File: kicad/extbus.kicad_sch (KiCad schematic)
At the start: 19 parts, among them J20 Spare resistors, J21 Power bar, J22 Spare resistors, J23 BUS Slot 2, J24 BUS Slot 1

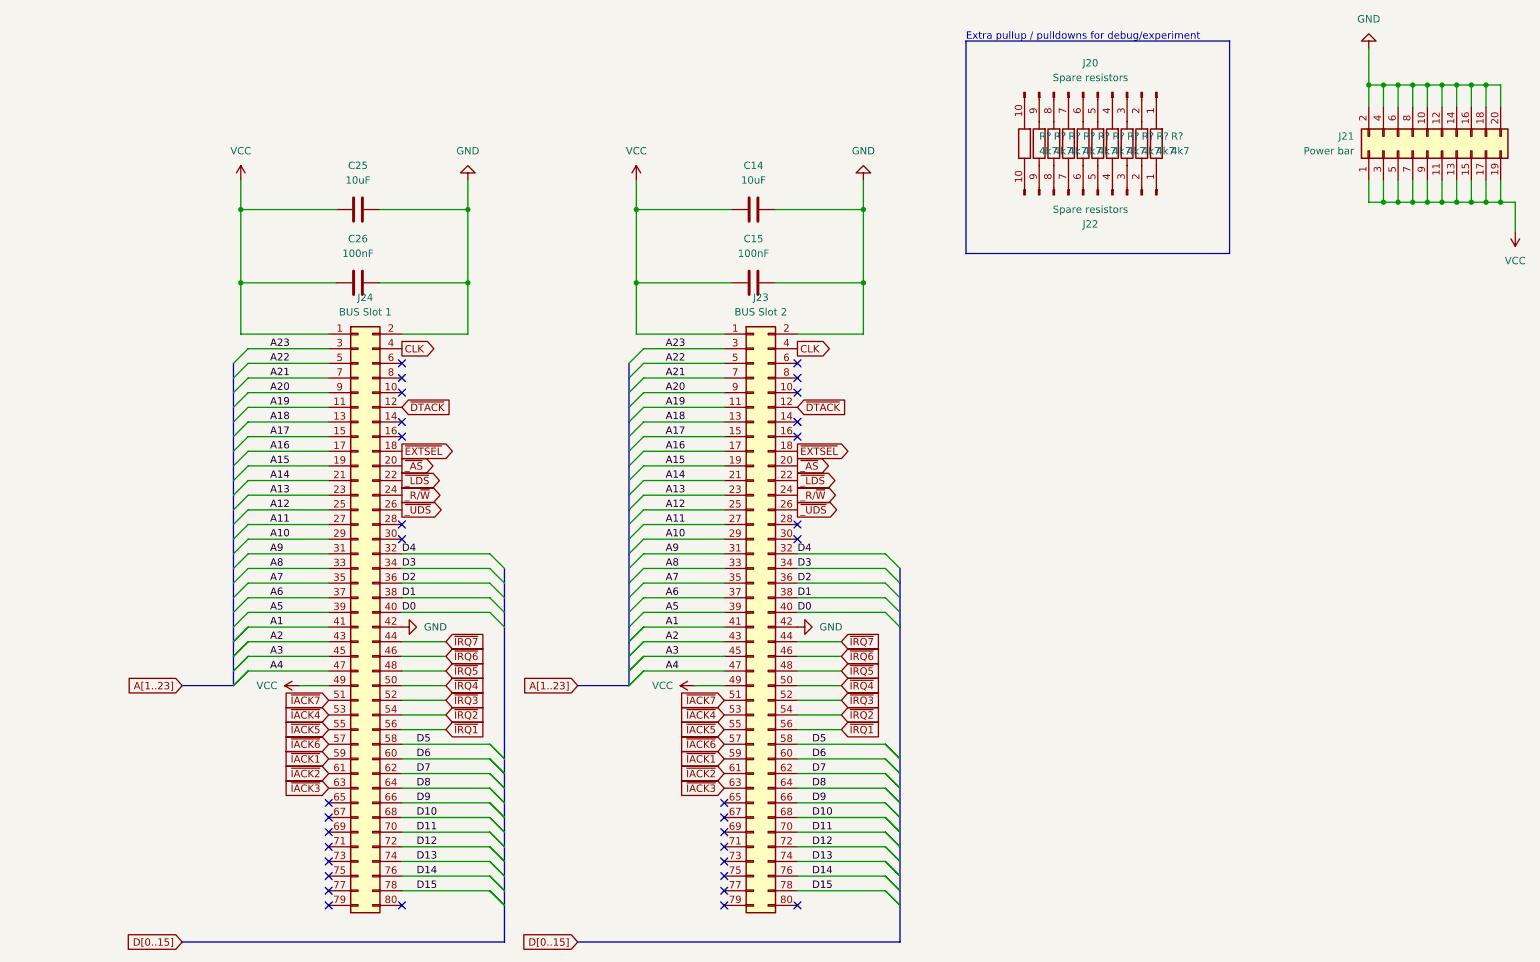
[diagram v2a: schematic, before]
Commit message: fiddlign with placement
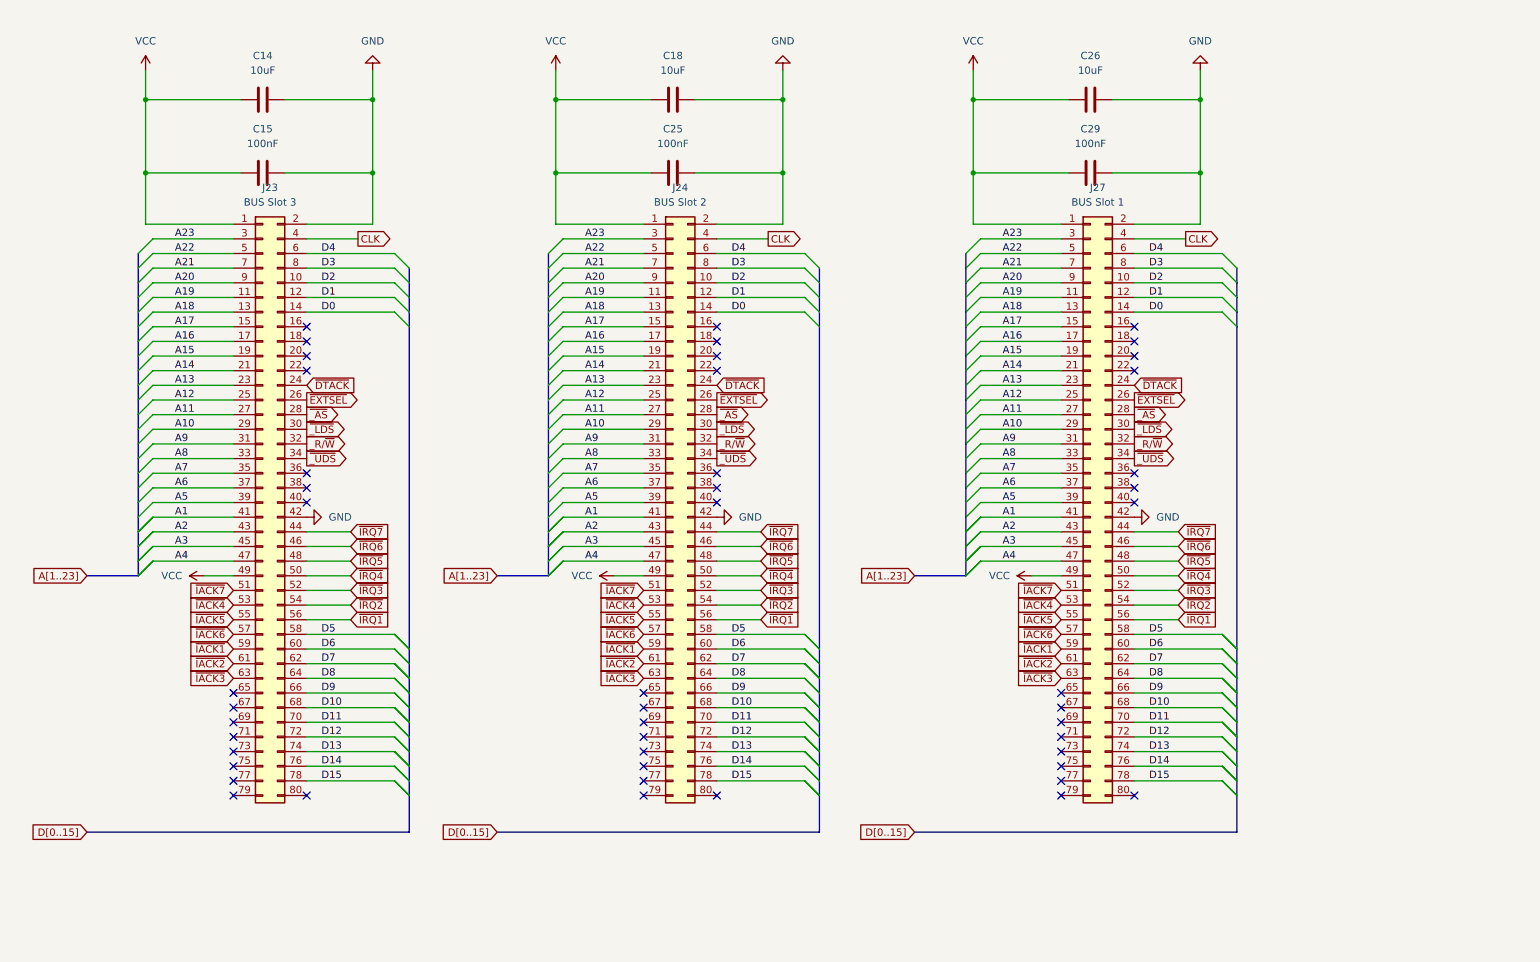
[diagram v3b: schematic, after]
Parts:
- removed J20, J22: Spare resistors, Connector_PinSocket_2.54mm:PinSocket_1x10_P2.54mm_Vertical, symbol Connector:Conn_01x10_Pin
- removed J21: Power bar, Connector_PinSocket_2.54mm:PinSocket_2x10_P2.54mm_Vertical, symbol Connector_Generic:Conn_02x10_Odd_Even
- removed R? (x10): 4k7, Resistor_THT:R_Axial_DIN0207_L6.3mm_D2.5mm_P10.16mm_Horizontal, symbol Device:R
- added C18: 10uF, Capacitor_THT:CP_Radial_D5.0mm_P2.50mm, symbol Device:C
- added C29: 100nF, Capacitor_THT:CP_Radial_D5.0mm_P2.50mm, symbol Device:C
- added J27: BUS Slot 1, Connector_PinSocket_2.54mm:PinSocket_2x40_P2.54mm_Vertical, symbol Connector_Generic:Conn_02x40_Odd_Even
- C25: value 10uF -> 100nF; footprint Capacitor_THT:C_Disc_D5.0mm_W2.5mm_P2.50mm -> Capacitor_THT:CP_Radial_D5.0mm_P2.50mm
- C26: value 100nF -> 10uF
- J23: value BUS Slot 2 -> BUS Slot 3
- J24: value BUS Slot 1 -> BUS Slot 2
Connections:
- net A1: now also J27.41 (Pin_41)
- net A10: now also J27.29 (Pin_29)
- net A11: now also J27.27 (Pin_27)
- net A12: now also J27.25 (Pin_25)
- net A13: now also J27.23 (Pin_23)
- net A14: now also J27.21 (Pin_21)
- net A15: now also J27.19 (Pin_19)
- net A16: now also J27.17 (Pin_17)
- net A17: now also J27.15 (Pin_15)
- net A18: now also J27.13 (Pin_13)
- net A19: now also J27.11 (Pin_11)
- net A2: now also J27.43 (Pin_43)
- net A20: now also J27.9 (Pin_9)
- net A21: now also J27.7 (Pin_7)
- net A22: now also J27.5 (Pin_5)
- net A23: now also J27.3 (Pin_3)
- net A3: now also J27.45 (Pin_45)
- net A4: now also J27.47 (Pin_47)
- net A5: now also J27.39 (Pin_39)
- net A6: now also J27.37 (Pin_37)
- net A7: now also J27.35 (Pin_35)
- net A8: now also J27.33 (Pin_33)
- net A9: now also J27.31 (Pin_31)
- net CLK: now also J27.4 (Pin_4)
- net D0: now also J23.14 (Pin_14), J24.14 (Pin_14), J27.14 (Pin_14); no longer J23.40 (Pin_40), J24.40 (Pin_40)
- net D1: now also J23.12 (Pin_12), J24.12 (Pin_12), J27.12 (Pin_12); no longer J23.38 (Pin_38), J24.38 (Pin_38)
- net D10: now also J27.68 (Pin_68)
- net D11: now also J27.70 (Pin_70)
- net D12: now also J27.72 (Pin_72)
- net D13: now also J27.74 (Pin_74)
- net D14: now also J27.76 (Pin_76)
- net D15: now also J27.78 (Pin_78)
- net D2: now also J23.10 (Pin_10), J24.10 (Pin_10), J27.10 (Pin_10); no longer J23.36 (Pin_36), J24.36 (Pin_36)
- net D3: now also J23.8 (Pin_8), J24.8 (Pin_8), J27.8 (Pin_8); no longer J23.34 (Pin_34), J24.34 (Pin_34)
- net D4: now also J23.6 (Pin_6), J24.6 (Pin_6), J27.6 (Pin_6); no longer J23.32 (Pin_32), J24.32 (Pin_32)
- net D5: now also J27.58 (Pin_58)
- net D6: now also J27.60 (Pin_60)
- net D7: now also J27.62 (Pin_62)
- net D8: now also J27.64 (Pin_64)
- net D9: now also J27.66 (Pin_66)
- net GND: now also C18.2, C29.2, J27.2 (Pin_2), J27.42 (Pin_42)
- net VCC: now also C18.1, C29.1, J27.1 (Pin_1), J27.49 (Pin_49)
- net _R/~{W}: now also J23.32 (Pin_32), J24.32 (Pin_32), J27.32 (Pin_32); no longer J23.24 (Pin_24), J24.24 (Pin_24)
- net ~{DTACK}: now also J23.24 (Pin_24), J24.24 (Pin_24), J27.24 (Pin_24); no longer J23.12 (Pin_12), J24.12 (Pin_12)
- net ~{EXTSEL}: now also J23.26 (Pin_26), J24.26 (Pin_26), J27.26 (Pin_26); no longer J23.18 (Pin_18), J24.18 (Pin_18)
- net ~{IACK1}: now also J27.59 (Pin_59)
- net ~{IACK2}: now also J27.61 (Pin_61)
- net ~{IACK3}: now also J27.63 (Pin_63)
- net ~{IACK4}: now also J27.53 (Pin_53)
- net ~{IACK5}: now also J27.55 (Pin_55)
- net ~{IACK6}: now also J27.57 (Pin_57)
- net ~{IACK7}: now also J27.51 (Pin_51)
- net ~{IRQ1}: now also J27.56 (Pin_56)
- net ~{IRQ2}: now also J27.54 (Pin_54)
- net ~{IRQ3}: now also J27.52 (Pin_52)
- net ~{IRQ4}: now also J27.50 (Pin_50)
- net ~{IRQ5}: now also J27.48 (Pin_48)
- net ~{IRQ6}: now also J27.46 (Pin_46)
- net ~{IRQ7}: now also J27.44 (Pin_44)
- net ~{_AS}: now also J23.28 (Pin_28), J24.28 (Pin_28), J27.28 (Pin_28); no longer J23.20 (Pin_20), J24.20 (Pin_20)
- net ~{_LDS}: now also J23.30 (Pin_30), J24.30 (Pin_30), J27.30 (Pin_30); no longer J23.22 (Pin_22), J24.22 (Pin_22)
- net ~{_UDS}: now also J23.34 (Pin_34), J24.34 (Pin_34), J27.34 (Pin_34); no longer J23.26 (Pin_26), J24.26 (Pin_26)
- no-connect marks 32 -> 48
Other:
- note removed: "Extra pullup / pulldowns for debug/experiment"
- moved on the sheet: C14, C15, J23
